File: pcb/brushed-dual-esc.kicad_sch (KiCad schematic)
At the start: 30 parts, among them J1 XT30PW-M, J2 TC2030-NL, J3 Conn_02x03_Odd_Even, J4 XT30PW-F, J5 XT30PW-F, U1 AZ1117-5.0, U2 TLV77133PDBVR, U3 STM32C011F4Ux, U4 DRV8231ADSGR, U5 DRV8231ADSGR

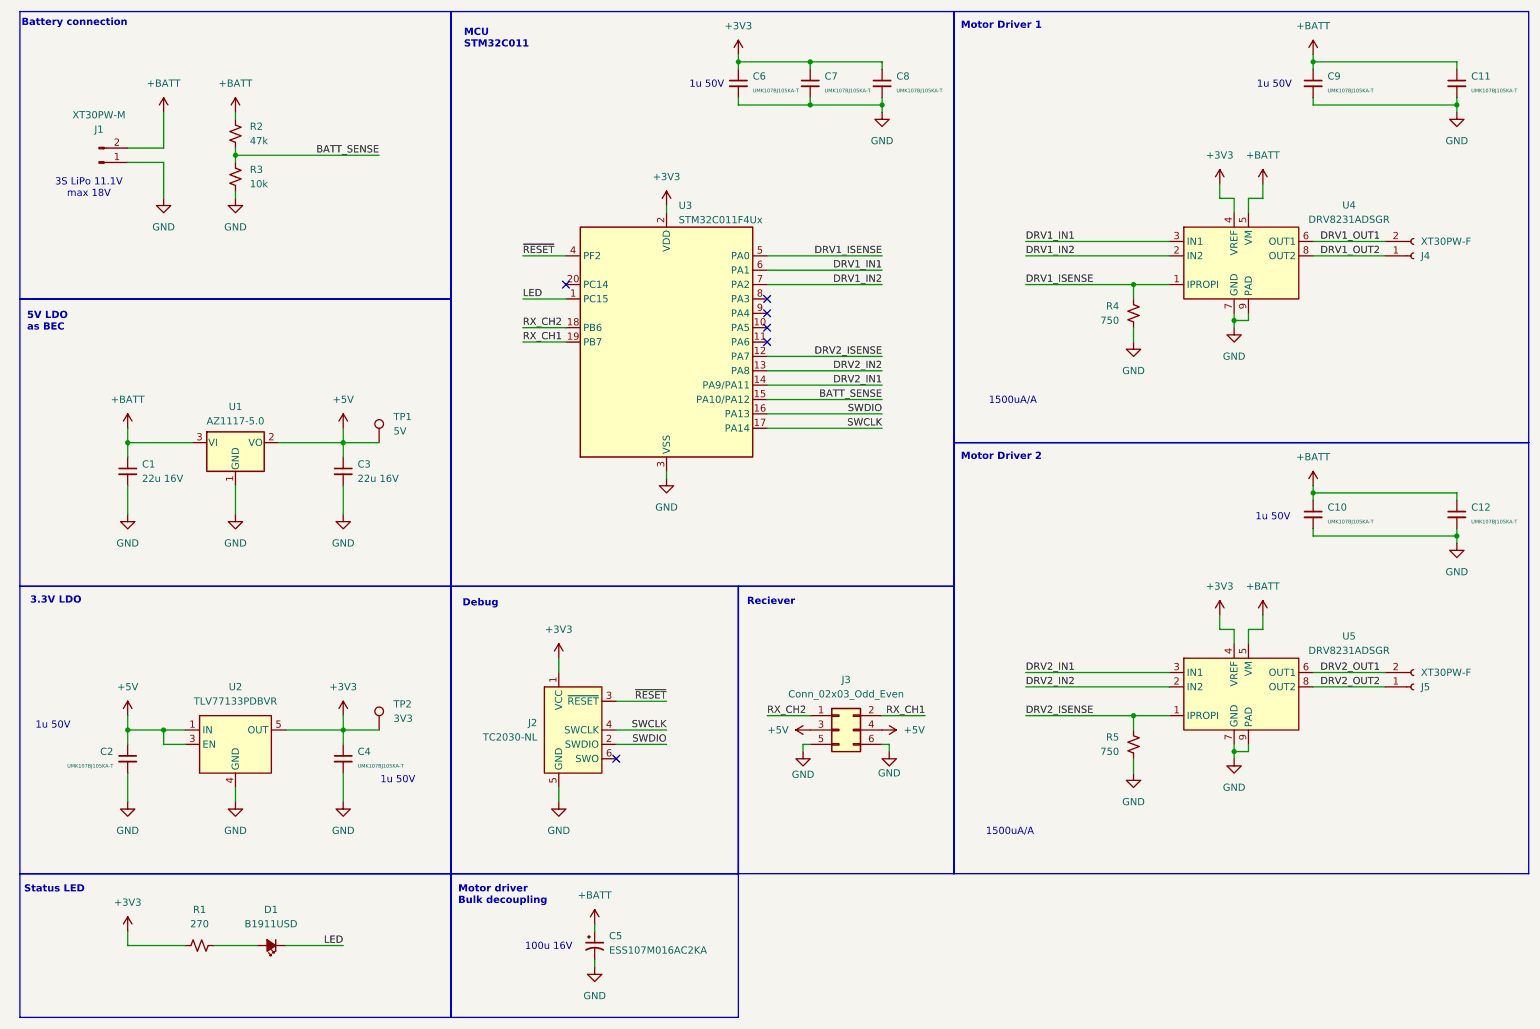
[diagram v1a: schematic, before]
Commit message: Schematic adjustment
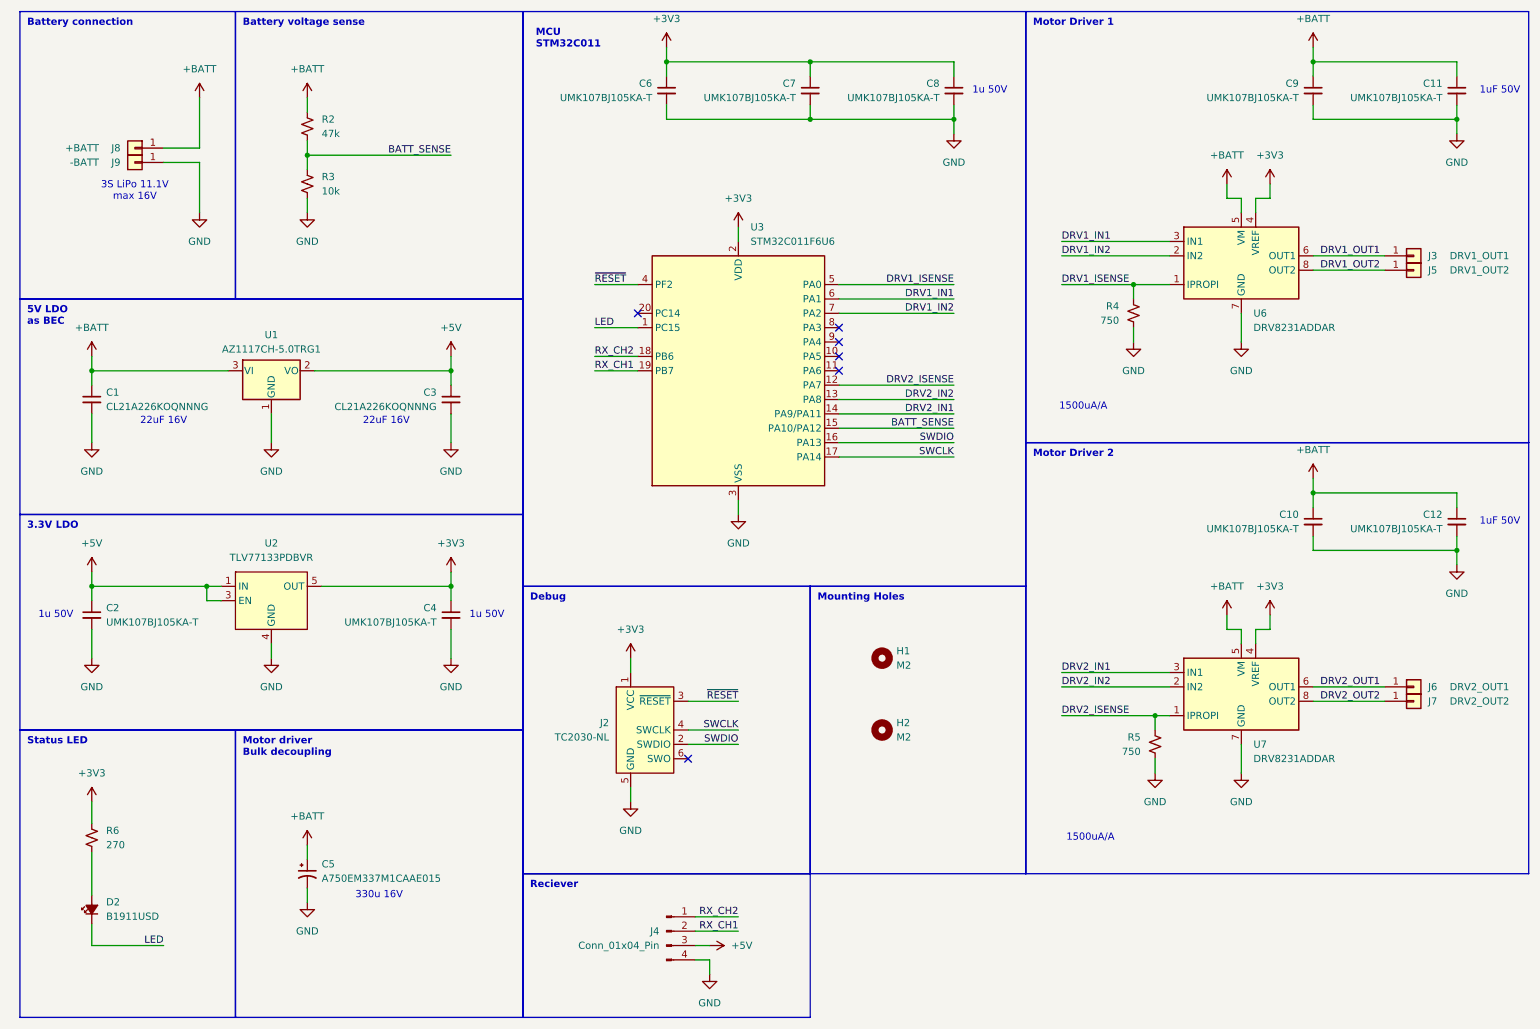
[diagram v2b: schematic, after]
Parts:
- removed D1: B1911USD, LED_SMD:LED_0603_1608Metric, symbol Device:LED_Small_Filled
- removed J1: XT30PW-M, Connector_AMASS:AMASS_XT30PW-M_1x02_P2.50mm_Horizontal, symbol Connector:Conn_01x02_Pin
- removed J3: Conn_02x03_Odd_Even, Connector_PinHeader_2.54mm:PinHeader_2x03_P2.54mm_Horizontal, symbol Connector_Generic:Conn_02x03_Odd_Even
- removed J4, J5: XT30PW-F, Connector_AMASS:AMASS_XT30PW-F_1x02_P2.50mm_Horizontal, symbol Connector:Conn_01x02_Socket
- removed R1: 270, Resistor_SMD:R_0603_1608Metric, symbol Device:R_Small_US
- removed TP1: 5V, TestPoint:TestPoint_Pad_D2.0mm, symbol Connector:TestPoint
- removed TP2: 3V3, TestPoint:TestPoint_Pad_D1.5mm, symbol Connector:TestPoint
- removed U4, U5: DRV8231ADSGR, Package_SON:WSON-8-1EP_2x2mm_P0.5mm_EP0.9x1.6mm, symbol Driver_Motor_TI:DRV8231ADSGR
- added D2: B1911USD, LED_SMD:LED_0603_1608Metric, symbol Device:LED_Small_Filled
- added H1, H2: M2, MountingHole:MountingHole_2.2mm_M2, symbol Mechanical:MountingHole
- added J3: DRV1_OUT1, Connector_Wire:SolderWirePad_1x01_SMD_2x4mm, symbol Connector_Generic:Conn_01x01
- added J4: Conn_01x04_Pin, Connector_PinHeader_2.54mm:PinHeader_1x04_P2.54mm_Vertical, symbol Connector:Conn_01x04_Pin
- added J5: DRV1_OUT2, Connector_Wire:SolderWirePad_1x01_SMD_2x4mm, symbol Connector_Generic:Conn_01x01
- added J6: DRV2_OUT1, Connector_Wire:SolderWirePad_1x01_SMD_2x4mm, symbol Connector_Generic:Conn_01x01
- added J7: DRV2_OUT2, Connector_Wire:SolderWirePad_1x01_SMD_2x4mm, symbol Connector_Generic:Conn_01x01
- added J8: +BATT, Connector_Wire:SolderWirePad_1x01_SMD_2x4mm, symbol Connector_Generic:Conn_01x01
- added J9: -BATT, Connector_Wire:SolderWirePad_1x01_SMD_2x4mm, symbol Connector_Generic:Conn_01x01
- added R6: 270, Resistor_SMD:R_0603_1608Metric, symbol Device:R_Small_US
- added U6, U7: DRV8231ADDAR, Package_SO:Texas_HSOP-8-1EP_3.9x4.9mm_P1.27mm, symbol Driver_Motor_TI:DRV8231ADDAR
- C1, C3: value 22u 16V -> CL21A226KOQNNNG; footprint Capacitor_SMD:C_0805_2012Metric -> Capacitor_SMD:C_1206_3216Metric
- C5: value ESS107M016AC2KA -> A750EM337M1CAAE015; footprint Capacitor_THT:CP_Radial_D5.0mm_P2.00mm -> Capacitor_THT:C_Radial_D6.3mm_H11.0mm_P2.50mm
- U1: value AZ1117-5.0 -> AZ1117CH-5.0TRG1
- U3: value STM32C011F4Ux -> STM32C011F6U6
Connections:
- net +3V3: now also R6.1, U6.4 (VREF), U7.4 (VREF)
- net +5V: now also J4.3 (Pin_3)
- net +BATT: now also J8.1 (Pin_1), U6.5 (VM), U7.5 (VM)
- net DRV1_IN1: now also U6.3 (IN1)
- net DRV1_IN2: now also U6.2 (IN2)
- net DRV1_ISENSE: now also U6.1 (IPROPI)
- net DRV1_OUT1: now also J3.1 (Pin_1), U6.6 (OUT1)
- net DRV1_OUT2: now also J5.1 (Pin_1), U6.8 (OUT2)
- net DRV2_IN1: now also U7.3 (IN1)
- net DRV2_IN2: now also U7.2 (IN2)
- net DRV2_ISENSE: now also U7.1 (IPROPI)
- net DRV2_OUT1: now also J6.1 (Pin_1), U7.6 (OUT1)
- net DRV2_OUT2: now also J7.1 (Pin_1), U7.8 (OUT2)
- net GND: now also J4.4 (Pin_4), J9.1 (Pin_1), U6.7 (GND), U6.9 (GND), U7.7 (GND), U7.9 (GND)
- net LED: now also D2.1 (K)
- net RX_CH1: now also J4.2 (Pin_2)
- net RX_CH2: now also J4.1 (Pin_1)
- new net: D2.2 (A), R6.2
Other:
- note added: "1uF 50V"
- note added: "22uF 16V"
- note added: "330u 16V"
- note added: "3S LiPo 11.1V max 16V"
- note added: "Battery voltage sense"
- note added: "Mounting Holes"
- note removed: "100u 16V"
- note removed: "3S LiPo 11.1V max 18V"
- moved on the sheet: C1, C10, C11, C12, C2, C3, C4, C5, C6, C7, C8, C9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
